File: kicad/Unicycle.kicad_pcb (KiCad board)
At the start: 2 copper layers, 120 x 120 mm, 19 parts, among them IC1 TSR 2 2450, P3 Battery Connector, P4 Safety Switch Connector, P5 Motor Driver Connector, P6 IMU Connector, U1 Teensy4.0

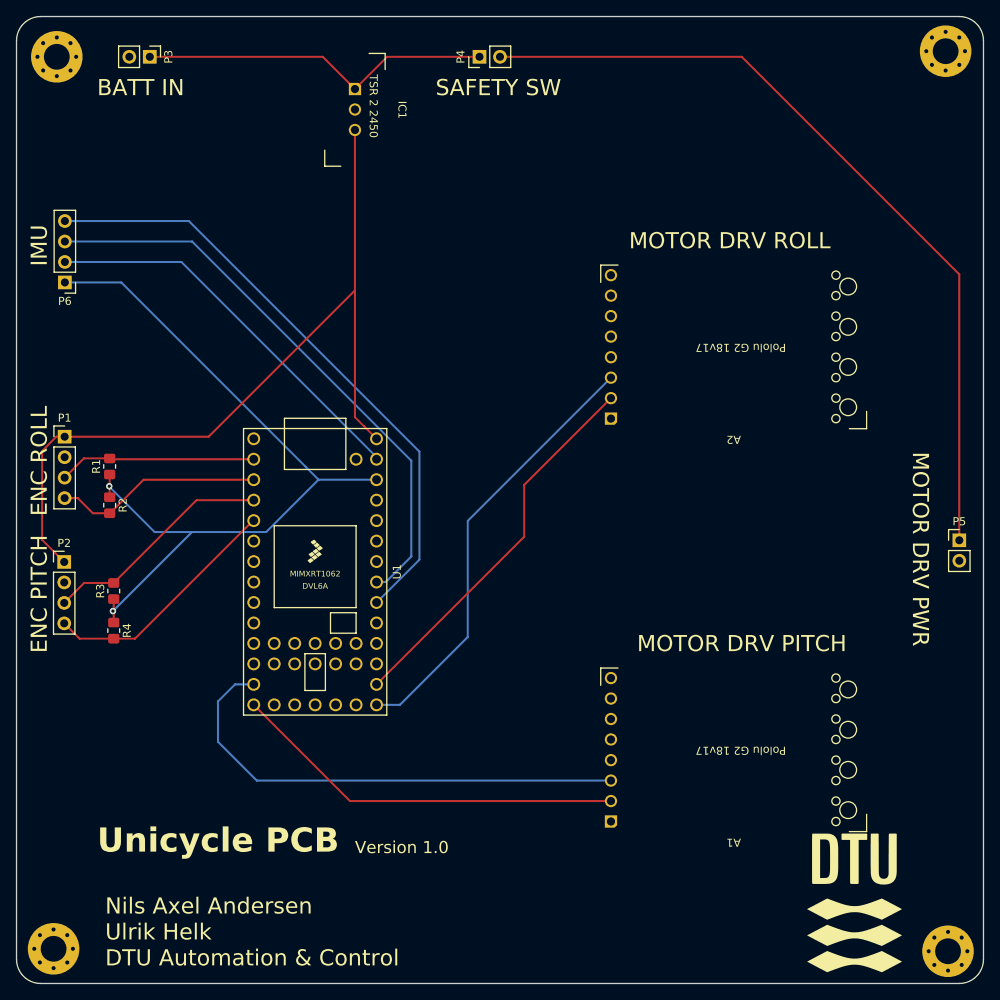
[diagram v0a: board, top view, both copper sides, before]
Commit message: update
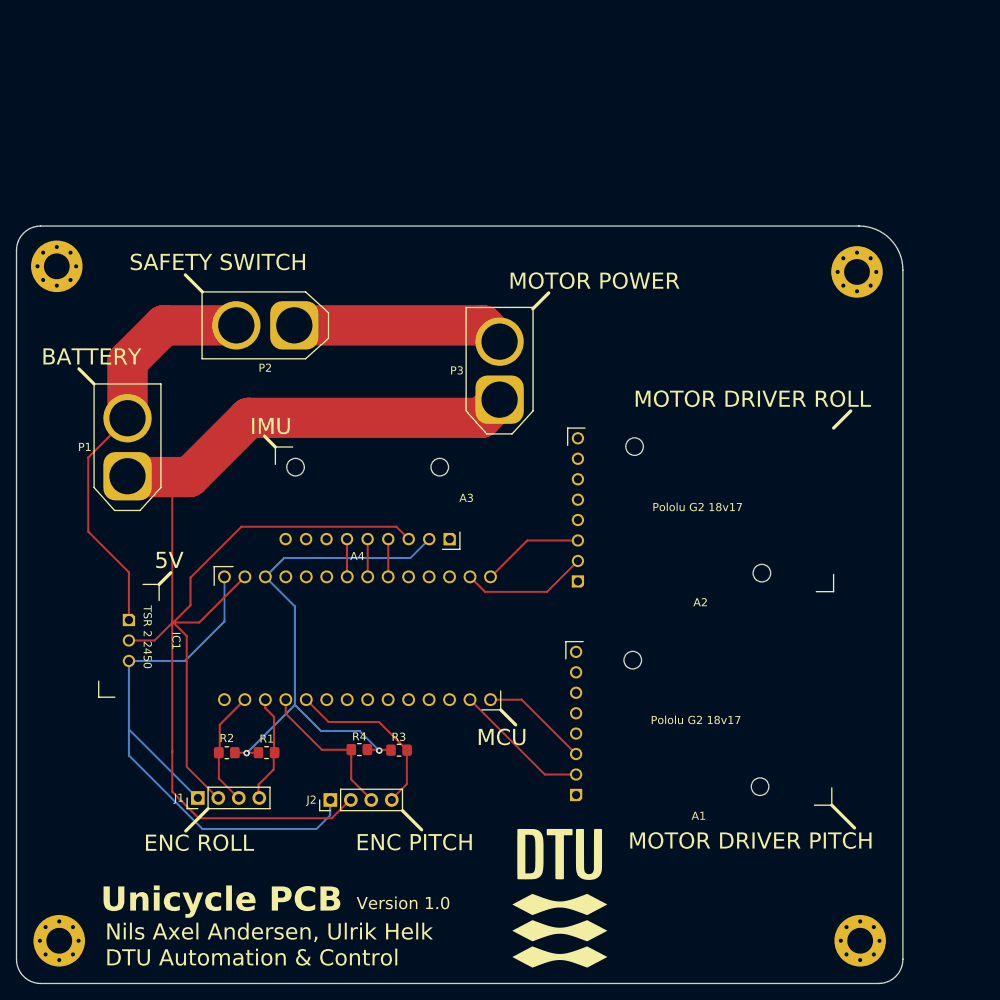
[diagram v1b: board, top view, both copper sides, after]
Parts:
- removed the P1 at (116.0, 102.1)
- removed the P2 at (115.9, 117.7)
- removed P6: IMU Connector, Connector_PinHeader_2.54mm:PinHeader_1x04_P2.54mm_Vertical
- removed U1: Teensy4.0, teensy_foot:Teensy40
- added A3: Pololu LSM6DSO, unicycle_foot:PololuLSM6DSO Text Up, F.Cu at (153.6, 109.8)
- added A4: Teensy 4.0, unicycle_foot:Teensy40 Simple, F.Cu at (152.3, 127.2)
- added J1: HEDS 5500 A, Connector_PinHeader_2.54mm:PinHeader_1x04_P2.54mm_Vertical, F.Cu at (132.5, 147.0)
- added J2: HEDS 5500 A, Connector_PinHeader_2.54mm:PinHeader_1x04_P2.54mm_Vertical, F.Cu at (148.9, 147.2)
- A1, A2: footprint unicycle_foot:Pololu G2 18v17 -> unicycle_foot:Pololu G2 18v17 Text Up
- P1: renamed from P3; footprint Connector_PinHeader_2.54mm:PinHeader_1x02_P2.54mm_Vertical -> Connector_AMASS:AMASS_XT60-F_1x02_P7.20mm_Vertical
- P2: renamed from P4; footprint Connector_PinHeader_2.54mm:PinHeader_1x02_P2.54mm_Vertical -> Connector_AMASS:AMASS_XT60-F_1x02_P7.20mm_Vertical
- P3: renamed from P5; footprint Connector_PinHeader_2.54mm:PinHeader_1x02_P2.54mm_Vertical -> Connector_AMASS:AMASS_XT60-F_1x02_P7.20mm_Vertical
- moved IC1 71.6 mm to (123.8, 127.5)
- moved P3 59.7 mm to (169.9, 97.5), turned to 90 degrees
- moved P1 52.1 mm to (123.8, 107.0), turned to 90 degrees
- moved R3 40.5 mm to (157.5, 141.1), turned to 0 degrees
- moved R1 40.5 mm to (141.0, 141.3), turned to 0 degrees
- moved P2 40.5 mm to (144.5, 88.3), turned to 180 degrees
- moved G*** 36.6 mm to (177.4, 159.4)
- moved R2 34.0 mm to (136.1, 141.4), turned to 180 degrees
- moved R4 33.9 mm to (152.6, 141.0), turned to 180 degrees
- moved H1 29.5 mm to (214.3, 81.7)
- moved H2 26.0 mm to (115.0, 81.0)
- moved A2 20.6 mm to (194.9, 111.2)
- moved H4 11.0 mm to (214.7, 164.7)
- moved A1 5.43 mm to (194.7, 137.7)
- moved H3 1.22 mm to (115.3, 164.7)
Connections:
- A1 pad 2: /DIRP -> DIR_ROLL
- A1 pad 3: /PWMP -> PWM_ROLL
- A2 pad 2: /PWMR -> DIR_PITCH
- A2 pad 3: /DIRR -> PWM_PITCH
- P1 pad 1: +BATT -> GND
- P1 pad 2: GND -> +BATT
- P2 pad 1: +BATT -> VM_LIM
- P2 pad 2: /VM_LIM -> +BATT
- P3 pad 1: /VM_LIM -> GND
- P3 pad 2: GND -> VM_LIM
- R1 pad 2: /AR -> ENC_B_ROLL
- R2 pad 2: /BR -> ENC_A_ROLL
- R3 pad 2: /AP -> ENC_B_PITCH
- R4 pad 2: /BP -> ENC_A_PITCH
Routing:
- net GND: track 49.0 -> 193.5 mm
- net /VM_LIM: track 101.2 -> 0.00 mm
- net /SDA: track 76.8 -> 0.00 mm
- net /SCL: track 71.8 -> 0.00 mm
- net /PWMP: track 61.1 -> 0.00 mm
- net /DIRR: track 54.3 -> 0.00 mm
- net /DIRP: track 49.3 -> 0.00 mm
- net /PWMR: track 47.6 -> 0.00 mm
- net +3.3V: track 99.8 -> 66.8 mm
- net /BP: track 30.4 -> 0.00 mm
- net /AP: track 28.8 -> 0.00 mm
- net +5V: track 101.4 -> 74.5 mm
- net VM_LIM: track 0.00 -> 26.3 mm
- net /BR: track 26.0 -> 0.00 mm
- net /AR: track 24.5 -> 0.00 mm
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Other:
- board size 120 x 120 mm -> 110 x 94 mm
- board text added: "5V"
- board text added: "BATTERY"
- board text added: "MCU"
- board text added: "MOTOR DRIVER PITCH"
- board text added: "MOTOR DRIVER ROLL"
- board text added: "MOTOR POWER"
- board text added: "Nils Axel Andersen, Ulrik Helk DTU Automation & Control"
- board text added: "SAFETY SWITCH"
- board text removed: "BATT IN"
- board text removed: "MOTOR DRV PITCH"
- board text removed: "MOTOR DRV PWR"
- board text removed: "MOTOR DRV ROLL"
- board text removed: "Nils Axel Andersen Ulrik Helk DTU Automation & Control"
- board text removed: "SAFETY SW"
